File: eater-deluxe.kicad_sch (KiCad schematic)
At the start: 7 parts, among them U1 6502, U2 W65C22NxP, U3 W65C51NxP, U4 28C256, U5 HM62256BLP, U6 CD74HC00E, U7 MXO45-3C-1M000000

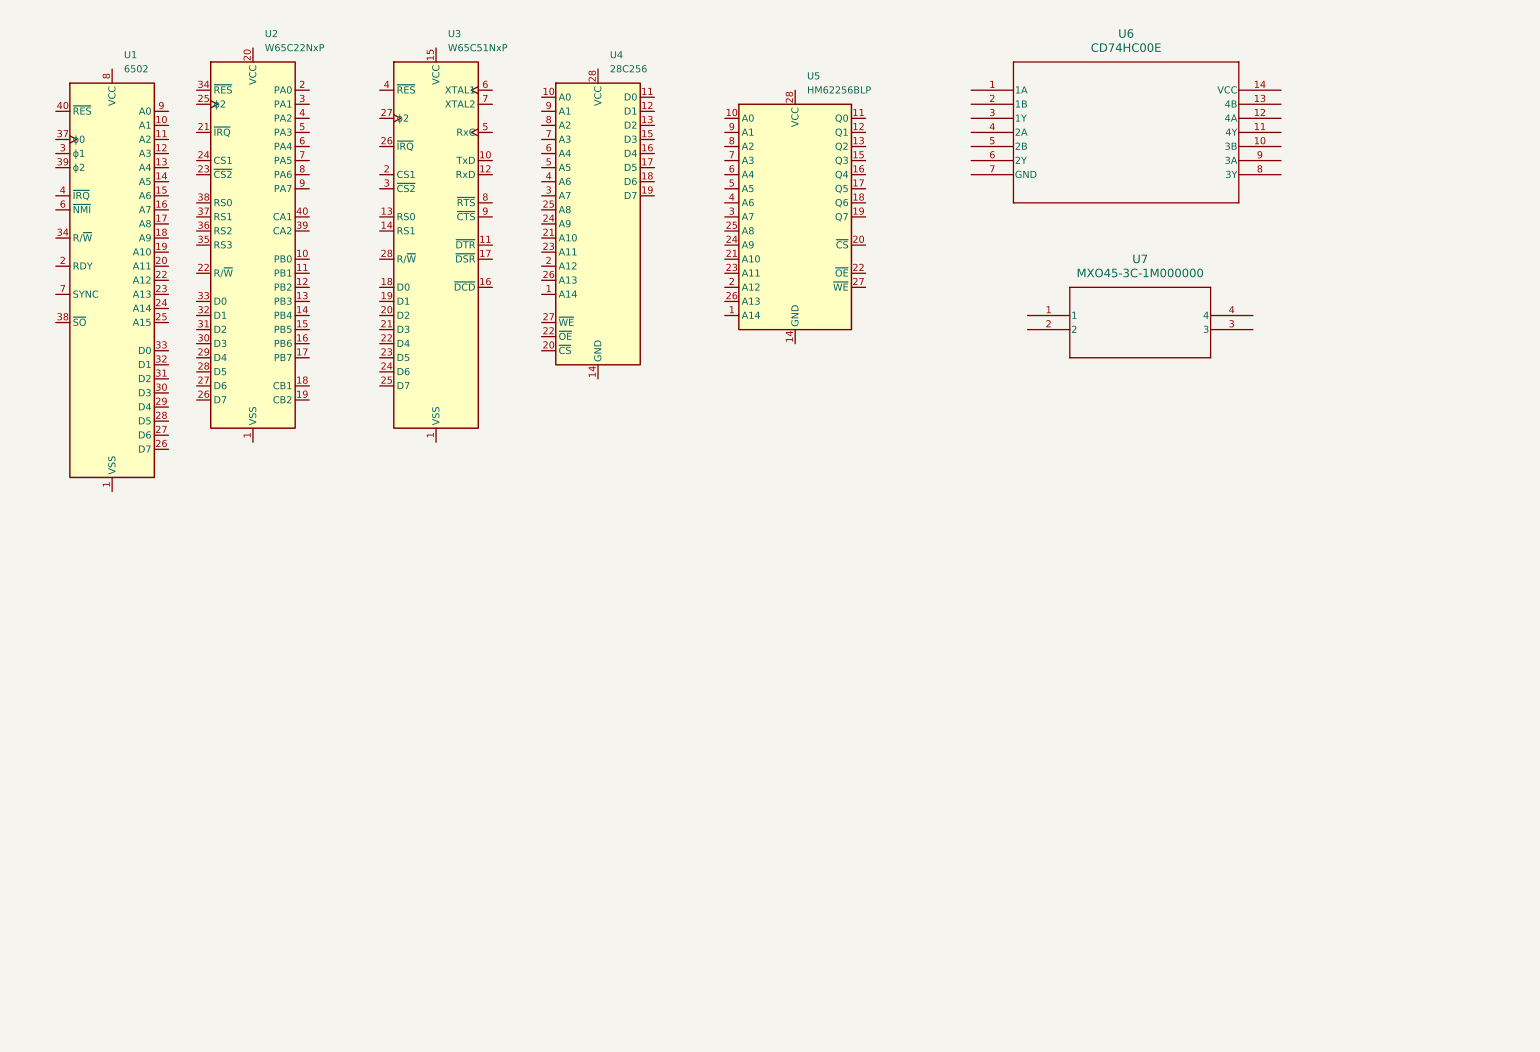
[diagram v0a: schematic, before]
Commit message: Schematics. Intermediate commit: only W65C22 Missing
Signed-off-by: Lucy <user@domain.tld>
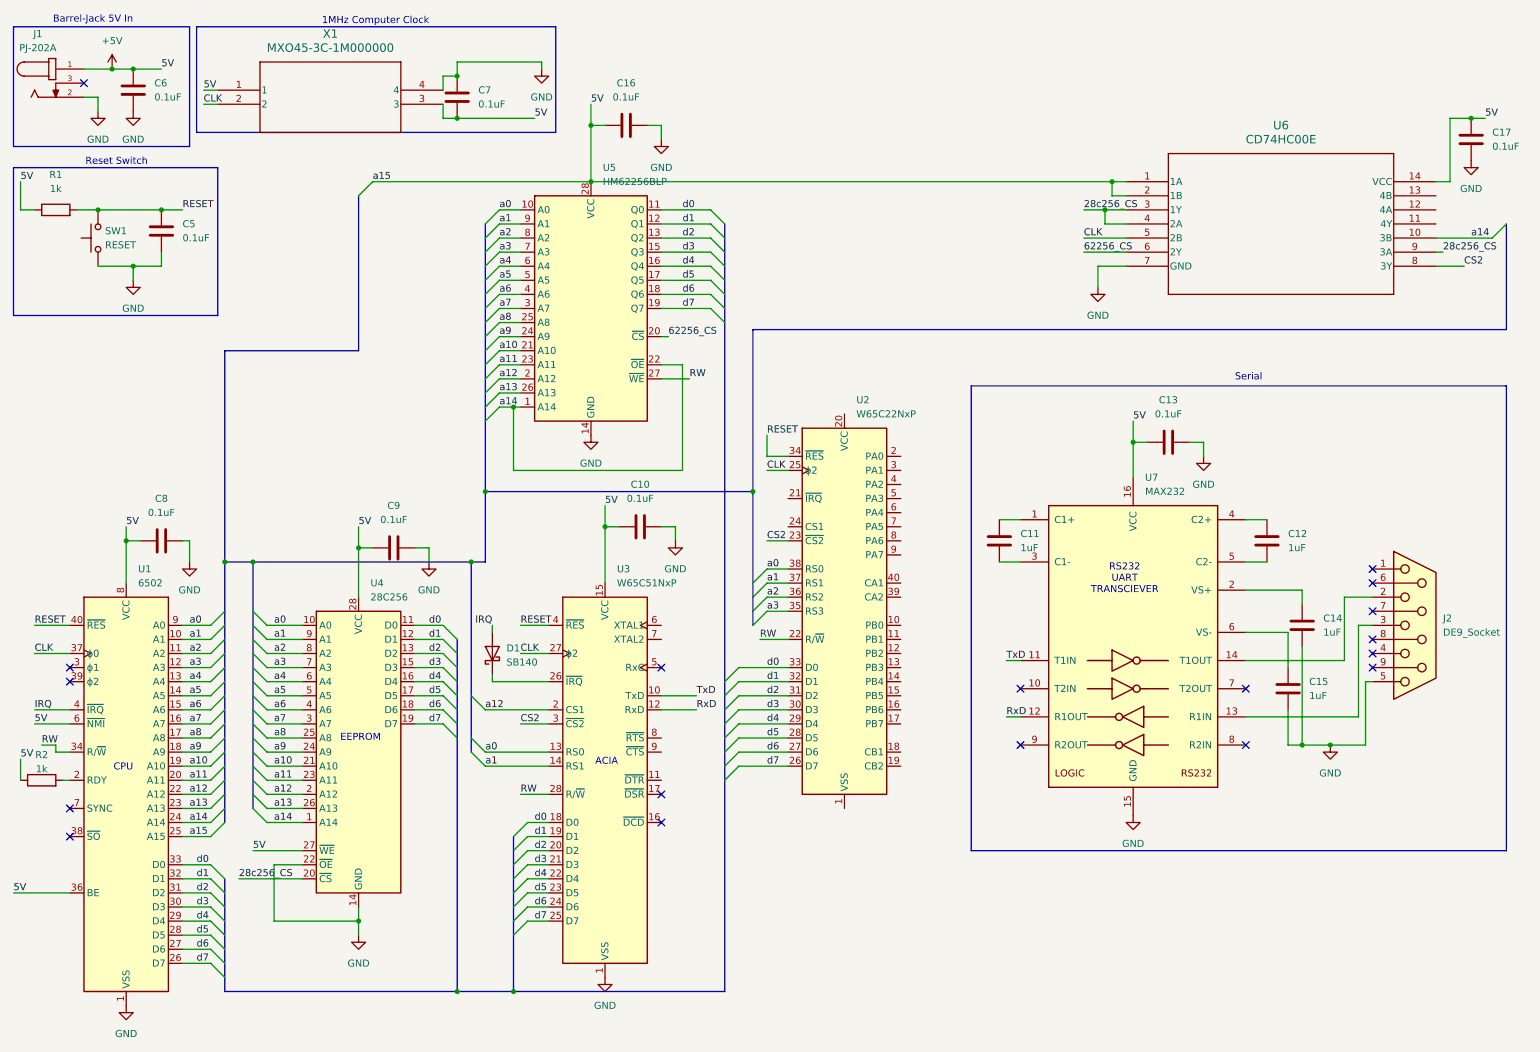
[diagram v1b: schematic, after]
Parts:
- added C10, C13, C16, C17, C5, C6, C7, C8, C9: 0.1uF, Capacitor_THT:C_Axial_L12.0mm_D6.5mm_P15.00mm_Horizontal, symbol Device:C
- added C11, C12, C14, C15: 1uF, Capacitor_THT:C_Axial_L12.0mm_D6.5mm_P15.00mm_Horizontal, symbol Device:C
- added D1: SB140, Diode_THT:D_DO-41_SOD81_P10.16mm_Horizontal, symbol Diode:SB140
- added J1: PJ-202A, PJ-202A:CUI_PJ-202A, symbol PJ-202A:PJ-202A
- added J2: DE9_Socket, Connector_Dsub:DSUB-9_Socket_Horizontal_P2.77x2.54mm_EdgePinOffset9.40mm, symbol Connector:DE9_Socket
- added R1, R2: 1k, Resistor_THT:R_Axial_DIN0204_L3.6mm_D1.6mm_P7.62mm_Horizontal, symbol Device:R
- added SW1: RESET, Button_Switch_THT:SW_PUSH-12mm, symbol Switch:SW_Push
- added U7: MAX232, Package_DIP:DIP-16_W7.62mm_Socket, symbol Interface_UART:MAX232
- renumbered U7 to X1
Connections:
- net GND: now reaches U3.1 (VSS)
- net GND: now also U1.1 (VSS), U1.21 (VSS), U4.14 (GND), U4.22 (~{OE}), U5.14 (GND), U6.7 (GND), X1.4, C10.2, C13.2, C14.2, C15.2, C16.2, C17.1, C5.1, C6.1, C7.2, C8.2, C9.2, J1.2, J2.5, SW1.1, U7.15 (GND)
- net TxD: now reaches U3.10 (TxD)
- net TxD: now also U7.11 (T1IN)
- net RxD: now reaches U3.12 (RxD)
- net RxD: now also U7.12 (R1OUT)
- net a0: now reaches U3.13 (RS0)
- net a0: now also U1.9 (A0), U2.38 (RS0), U4.10 (A0), U5.10 (A0)
- net a1: now reaches U3.14 (RS1)
- net a1: now also U1.10 (A1), U2.37 (RS1), U4.9 (A1), U5.9 (A1)
- net +5V: now reaches U3.15 (VCC)
- net +5V: now also U1.25 (A15), U1.36 (BE), U1.6 (~{NMI}), U1.8 (VCC), U4.27 (~{WE}), U4.28 (VCC), U5.28 (VCC), U6.1 (1A), U6.14 (VCC), U6.2 (1B), X1.1, X1.3, C10.1, C13.1, C16.1, C17.2, C6.2, C7.1, C8.1, C9.1, J1.1, R1.1, R2.1, U7.16 (VCC)
- net d0: now reaches U3.18 (D0)
- net d0: now also U1.33 (D0), U2.33 (D0), U4.11 (D0), U5.11 (Q0)
- net d1: now reaches U3.19 (D1)
- net d1: now also U1.32 (D1), U2.32 (D1), U4.12 (D1), U5.12 (Q1)
- net a12: now reaches U3.2 (CS1)
- net a12: now also U1.22 (A12), U4.2 (A12), U5.2 (A12)
- net d2: now reaches U3.20 (D2)
- net d2: now also U1.31 (D2), U2.31 (D2), U4.13 (D2), U5.13 (Q2)
- net d3: now reaches U3.21 (D3)
- net d3: now also U1.30 (D3), U2.30 (D3), U4.15 (D3), U5.15 (Q3)
- net d4: now reaches U3.22 (D4)
- net d4: now also U1.29 (D4), U2.29 (D4), U4.16 (D4), U5.16 (Q4)
- net d5: now reaches U3.23 (D5)
- net d5: now also U1.28 (D5), U2.28 (D5), U4.17 (D5), U5.17 (Q5)
- net d6: now reaches U3.24 (D6)
- net d6: now also U1.27 (D6), U2.27 (D6), U4.18 (D6), U5.18 (Q6)
- net d7: now reaches U3.25 (D7)
- net d7: now also U1.26 (D7), U2.26 (D7), U4.19 (D7), U5.19 (Q7)
- net at U3.26 (~{IRQ}): now also D1.1 (K)
- net CLK: now reaches U3.27 (ϕ2)
- net CLK: now also U1.37 (ϕ0), U2.25 (ϕ2), U6.5 (2B), X1.2
- net RW: now reaches U3.28 (R/~{W})
- net RW: now also U1.34 (R/~{W}), U2.22 (R/~{W}), U5.27 (~{WE})
- net CS2: now reaches U3.3 (~{CS2})
- net CS2: now also U2.23 (~{CS2}), U6.8 (3Y)
- net RESET: now reaches U3.4 (~{RES})
- net RESET: now also U1.40 (~{RES}), U2.34 (~{RES}), C5.2, R1.2, SW1.2
- net a14: now reaches U5.1 (A14)
- net a14: now also U1.24 (A14), U4.1 (A14), U5.22 (~{OE}), U6.10 (3B)
- net 62256_CS: now reaches U5.20 (~{CS})
- net 62256_CS: now also U6.6 (2Y)
- net a10: now reaches U5.21 (A10)
- net a10: now also U1.19 (A10), U4.21 (A10)
- net a11: now reaches U5.23 (A11)
- net a11: now also U1.20 (A11), U4.23 (A11)
- net a9: now reaches U5.24 (A9)
- net a9: now also U1.18 (A9), U4.24 (A9)
- net a8: now reaches U5.25 (A8)
- net a8: now also U1.17 (A8), U4.25 (A8)
- net a13: now reaches U5.26 (A13)
- net a13: now also U1.23 (A13), U4.26 (A13)
- net a7: now reaches U5.3 (A7)
- net a7: now also U1.16 (A7), U4.3 (A7)
- net a6: now reaches U5.4 (A6)
- net a6: now also U1.15 (A6), U4.4 (A6)
- net a5: now reaches U5.5 (A5)
- net a5: now also U1.14 (A5), U4.5 (A5)
- net a4: now reaches U5.6 (A4)
- net a4: now also U1.13 (A4), U4.6 (A4)
- net a3: now reaches U5.7 (A3)
- net a3: now also U1.12 (A3), U2.35 (RS3), U4.7 (A3)
- net a2: now reaches U5.8 (A2)
- net a2: now also U1.11 (A2), U2.36 (RS2), U4.8 (A2)
- net 28c256_CS: now reaches U4.20 (~{CS})
- net 28c256_CS: now also U6.3 (1Y), U6.4 (2A), U6.9 (3A)
- net at U1.2 (RDY): now also R2.2
- net IRQ: now reaches U1.4 (~{IRQ})
- net IRQ: now also D1.2 (A)
- new net: J2.2, U7.14 (T1OUT)
- new net: J2.3, U7.13 (R1IN)
- new net: C14.1, U7.2 (VS+)
- new net: C11.1, U7.1 (C1+)
- new net: C11.2, U7.3 (C1-)
- new net: C15.1, U7.6 (VS-)
- new net: C12.1, U7.4 (C2+)
- new net: C12.2, U7.5 (C2-)
- no-connect marks 0 -> 18
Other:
- note added: "1MHz Computer Clock"
- note added: "ACIA"
- note added: "Barrel-Jack 5V In"
- note added: "CPU"
- note added: "EEPROM"
- note added: "RS232 UART TRANSCIEVER"
- note added: "Reset Switch"
- note added: "Serial"
- moved on the sheet: U2, U3, U4, U5, U6, X1
